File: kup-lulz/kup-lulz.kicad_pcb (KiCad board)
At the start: 4 copper layers, 144.5 x 137 mm, 229 parts, among them J1 CONN_PCIE_PWR_8PIN, J10 SFP_CAGE, J11 CONN_SFP_HOST, J12 SFP_CAGE, J13 PMOD_HOST, J14 PMOD_HOST, J15 CONN_QSFP_HOST, J16 CONN_QSFP_HOST, J17 SMPM, J18 SMPM, J19 SMPM, J2 CONN_IBC_MGMT, J20 SMPM, J21 SMPM, J22 SMPM, J23 SMPM, J24 SMPM, J25 SMPM, J26 SMPM, J27 SMPM, J28 SMPM, J29 SMPM, J3 CONN_01X03, J30 SMPM, J31 SMPM, J32 SMPM, J33 CONN_SFP_HOST, J34 SFP_CAGE, J35 QSFP_CAGE, J36 QSFP_CAGE, J4 CONN_01X05, J7 CONN_SFP_HOST, J8 SFP_CAGE, J9 CONN_SFP_HOST, M1 HEATSINK, M2 SCREWHOLE, M3 SCREWHOLE, M4 SCREWHOLE, M5 SCREWHOLE, SW1 SWITCH, SW2 SWITCH, U1 STM32L031C6U6, U2 MYMGK1R812ERSR, U3 MYMGK1R812ERSR, U4 MYMGK00506ERSR, U5 MYMGK00504ERSR, U6 MYMGK00504ERSR, U7 MYMGK00504ERSR, U9 XILINX_ULTRASCALEPLUS_B676

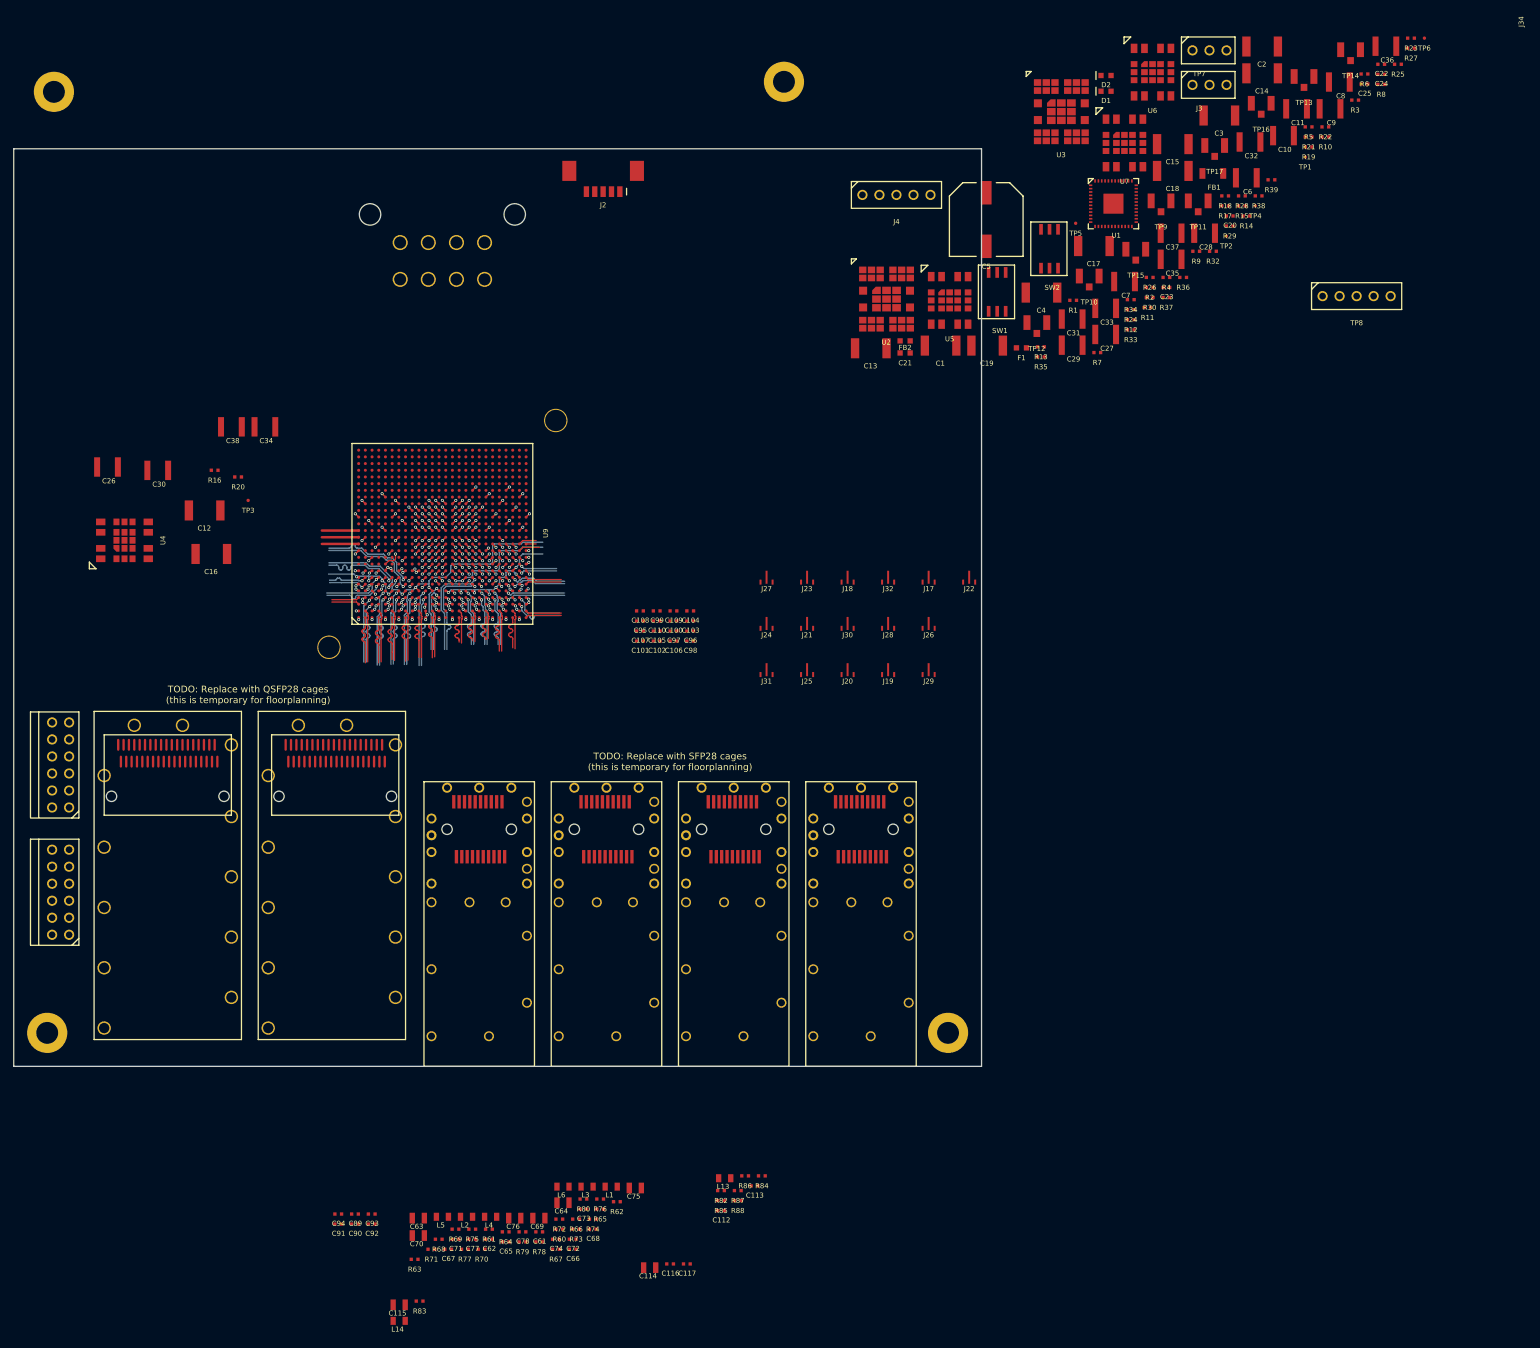
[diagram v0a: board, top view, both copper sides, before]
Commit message: Continued initial work on kup-lulz devboard
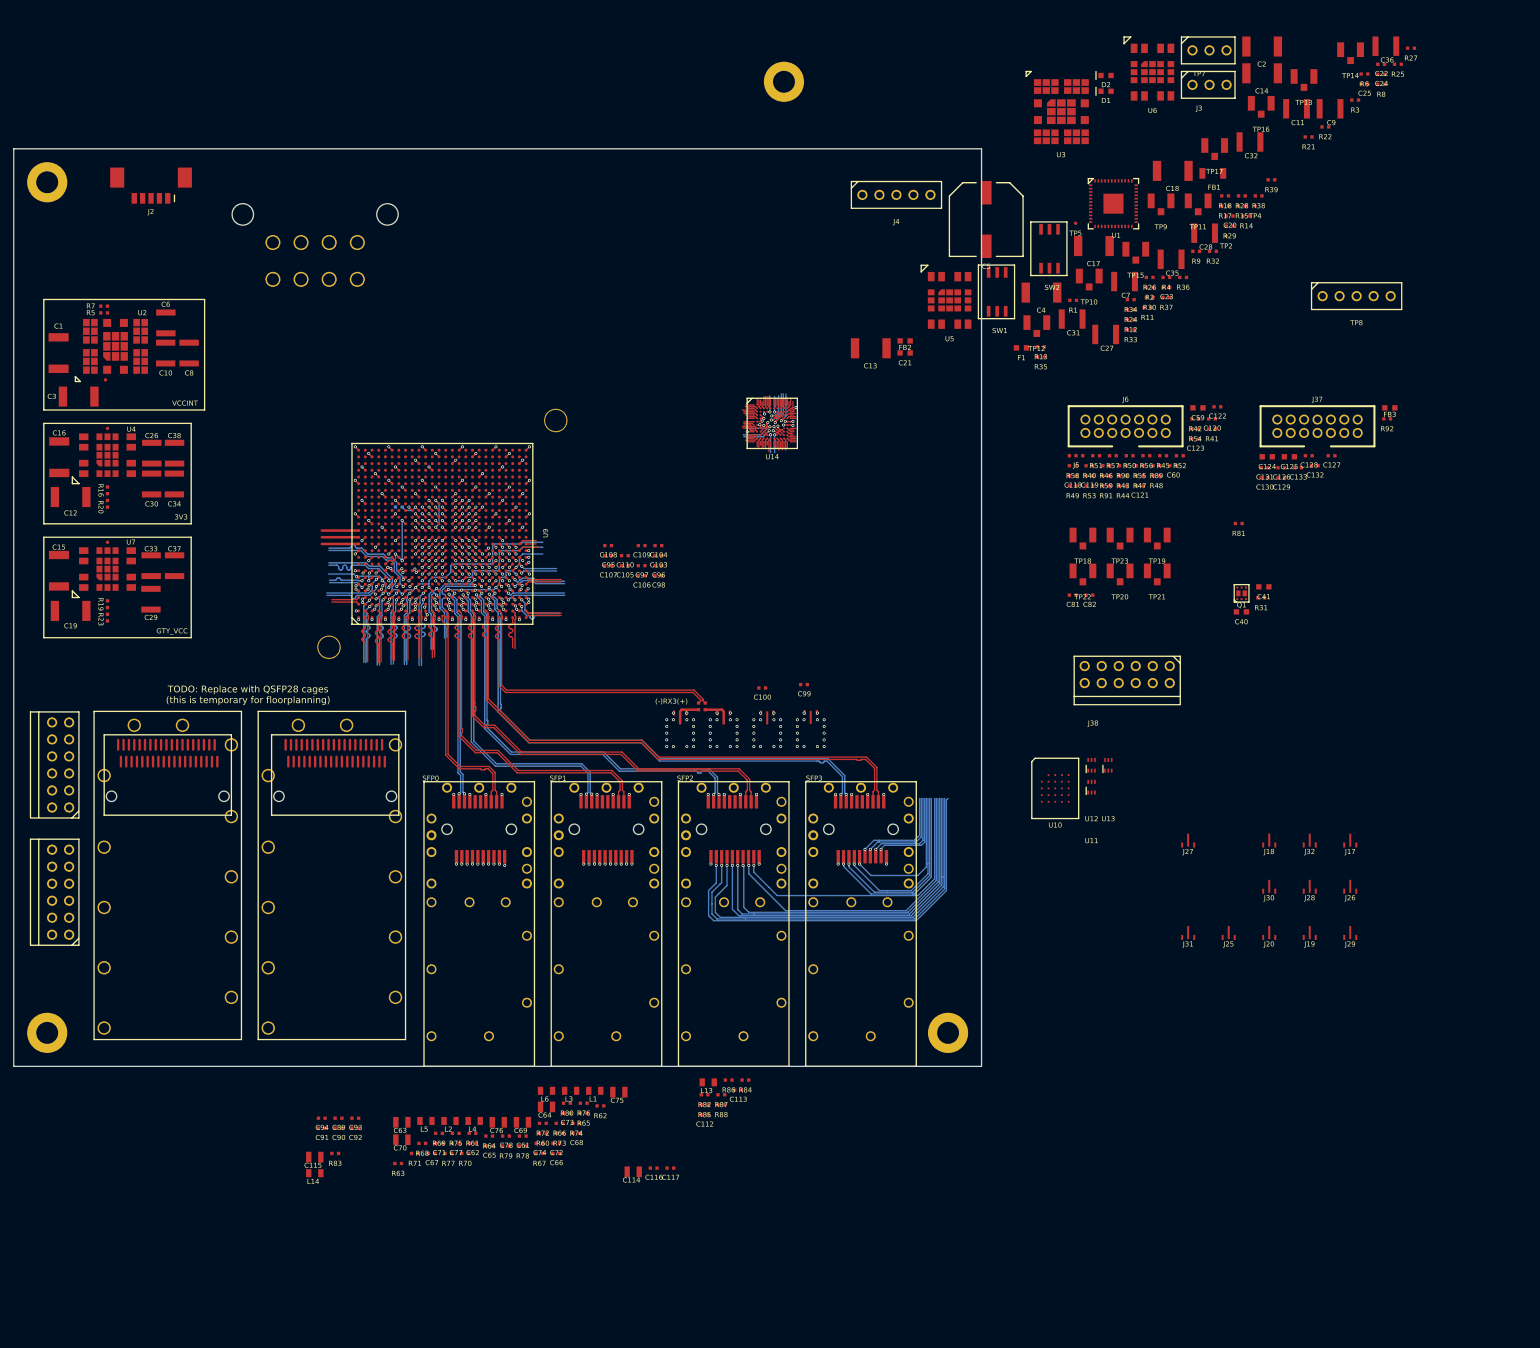
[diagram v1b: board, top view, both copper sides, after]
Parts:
- added C118: 0.47 uF, azonenberg_pcb:EIA_0402_CAP_NOSILK, F.Cu at (208.6, 82.8)
- added C119: 0.47 uF, azonenberg_pcb:EIA_0402_CAP_NOSILK, F.Cu at (211.1, 82.8)
- added C120: 0.47 uF, azonenberg_pcb:EIA_0402_CAP_NOSILK, F.Cu at (229.4, 74.3)
- added C121: 0.47 uF, azonenberg_pcb:EIA_0402_CAP_NOSILK, F.Cu at (218.6, 84.3)
- added C122: 0.47 uF, azonenberg_pcb:EIA_0402_CAP_NOSILK, F.Cu at (230.2, 72.5)
- added C123: 0.47 uF, azonenberg_pcb:EIA_0402_CAP_NOSILK, F.Cu at (226.9, 77.3)
- added C124: 4.7 uF, azonenberg_pcb:EIA_0603_CAP_NOSILK, F.Cu at (237.7, 80.0)
- added C125: 4.7 uF, azonenberg_pcb:EIA_0603_CAP_NOSILK, F.Cu at (241.0, 80.0)
- added C126: 0.47 uF, azonenberg_pcb:EIA_0402_CAP_NOSILK, F.Cu at (239.8, 81.6)
- added C127: 0.47 uF, azonenberg_pcb:EIA_0402_CAP_NOSILK, F.Cu at (247.3, 79.8)
- added C128: 0.47 uF, azonenberg_pcb:EIA_0402_CAP_NOSILK, F.Cu at (243.9, 79.8)
- added C129: 0.47 uF, azonenberg_pcb:EIA_0402_CAP_NOSILK, F.Cu at (239.8, 83.1)
- added C130: 0.47 uF, azonenberg_pcb:EIA_0402_CAP_NOSILK, F.Cu at (237.3, 83.1)
- added C131: 0.47 uF, azonenberg_pcb:EIA_0402_CAP_NOSILK, F.Cu at (237.3, 81.6)
- added C132: 0.47 uF, azonenberg_pcb:EIA_0402_CAP_NOSILK, F.Cu at (244.8, 81.3)
- added C133: 0.47 uF, azonenberg_pcb:EIA_0402_CAP_NOSILK, F.Cu at (242.3, 81.6)
- added C40: 4.7 uF, azonenberg_pcb:EIA_0603_CAP_NOSILK, F.Cu at (233.8, 103.2)
- added C41: 4.7 uF, azonenberg_pcb:EIA_0603_CAP_NOSILK, F.Cu at (237.2, 99.4)
- added C59: 4.7 uF, azonenberg_pcb:EIA_0603_CAP_NOSILK, F.Cu at (227.3, 72.7)
- added C60: 0.47 uF, azonenberg_pcb:EIA_0402_CAP_NOSILK, F.Cu at (223.6, 81.3)
- added C81: 0.1 uF, azonenberg_pcb:EIA_0402_CAP_NOSILK, F.Cu at (208.6, 100.7)
- added C82: 0.1 uF, azonenberg_pcb:EIA_0402_CAP_NOSILK, F.Cu at (211.1, 100.7)
- added FB3: MI0603J601R-10, azonenberg_pcb:EIA_0603_INDUCTOR_NOSILK, F.Cu at (256.0, 72.7)
- added J37: XILINX_JTAG, azonenberg_pcb:XILINX_JTAG_PTH_MOLEX_0878311420, F.Cu at (245.2, 75.4)
- added J38: PMOD_HOST, azonenberg_pcb:CONN_HEADER_2.54MM_2x6_RA_PMOD_HOST, F.Cu at (216.8, 112.5)
- added J5: JUMPER_0402, azonenberg_pcb:EIA_0402_JUMPER, F.Cu at (209.1, 79.8)
- added J6: XILINX_JTAG, azonenberg_pcb:XILINX_JTAG_PTH_MOLEX_0878311420, F.Cu at (216.5, 75.4)
- added Q1: SSM6N58NU, azonenberg_pcb:DFN_6_0.65MM_2x2MM_GDS, F.Cu at (233.8, 100.4)
- added R31: 1K, azonenberg_pcb:EIA_0402_RES_NOSILK, F.Cu at (236.8, 101.0)
- added R40: 0, azonenberg_pcb:EIA_0402_RES_NOSILK, F.Cu at (211.1, 81.3)
- added R41: 0, azonenberg_pcb:EIA_0402_RES_NOSILK, F.Cu at (229.4, 75.8)
- added R42: 0, azonenberg_pcb:EIA_0402_RES_NOSILK, F.Cu at (226.9, 74.3)
- added R43: 4.7K, azonenberg_pcb:EIA_0402_RES_NOSILK, F.Cu at (216.1, 82.8)
- added R44: 33, azonenberg_pcb:EIA_0402_RES_NOSILK, F.Cu at (216.1, 84.3)
- added R45: 33, azonenberg_pcb:EIA_0402_RES_NOSILK, F.Cu at (222.1, 79.8)
- added R46: 33, azonenberg_pcb:EIA_0402_RES_NOSILK, F.Cu at (213.6, 81.3)
- added R47: 33, azonenberg_pcb:EIA_0402_RES_NOSILK, F.Cu at (218.6, 82.8)
- added R48: 33, azonenberg_pcb:EIA_0402_RES_NOSILK, F.Cu at (221.1, 82.8)
- added R49: 33, azonenberg_pcb:EIA_0402_RES_NOSILK, F.Cu at (208.6, 84.3)
- added R50: 33, azonenberg_pcb:EIA_0402_RES_NOSILK, F.Cu at (217.1, 79.8)
- added R51: 33, azonenberg_pcb:EIA_0402_RES_NOSILK, F.Cu at (212.1, 79.8)
- added R52: 33, azonenberg_pcb:EIA_0402_RES_NOSILK, F.Cu at (224.6, 79.8)
- added R53: 33, azonenberg_pcb:EIA_0402_RES_NOSILK, F.Cu at (211.1, 84.3)
- added R54: 33, azonenberg_pcb:EIA_0402_RES_NOSILK, F.Cu at (226.9, 75.8)
- added R55: 4.7K, azonenberg_pcb:EIA_0402_RES_NOSILK, F.Cu at (218.6, 81.3)
- added R56: 4.7K, azonenberg_pcb:EIA_0402_RES_NOSILK, F.Cu at (219.6, 79.8)
- added R57: 4.7K, azonenberg_pcb:EIA_0402_RES_NOSILK, F.Cu at (214.6, 79.8)
- added R58: 4.7K, azonenberg_pcb:EIA_0402_RES_NOSILK, F.Cu at (208.6, 81.3)
- added R59: 4.7K, azonenberg_pcb:EIA_0402_RES_NOSILK, F.Cu at (213.6, 82.8)
- added R81: 100, azonenberg_pcb:EIA_0402_RES_NOSILK, F.Cu at (233.4, 90.0)
- added R89: 4.7K, azonenberg_pcb:EIA_0402_RES_NOSILK, F.Cu at (221.1, 81.3)
- added R90: 4.7K, azonenberg_pcb:EIA_0402_RES_NOSILK, F.Cu at (216.1, 81.3)
- added R91: 4.7K, azonenberg_pcb:EIA_0402_RES_NOSILK, F.Cu at (213.6, 84.3)
- added R92: 33, azonenberg_pcb:EIA_0402_RES_NOSILK, F.Cu at (255.6, 74.3)
- added TP18: U.FL, azonenberg_pcb:CONN_U.FL_TE_1909763-1, F.Cu at (210.1, 91.8)
- added TP19: U.FL, azonenberg_pcb:CONN_U.FL_TE_1909763-1, F.Cu at (221.2, 91.8)
- added TP20: U.FL, azonenberg_pcb:CONN_U.FL_TE_1909763-1, F.Cu at (215.7, 97.1)
- added TP21: U.FL, azonenberg_pcb:CONN_U.FL_TE_1909763-1, F.Cu at (221.2, 97.1)
- added TP22: U.FL, azonenberg_pcb:CONN_U.FL_TE_1909763-1, F.Cu at (210.1, 97.1)
- added TP23: U.FL, azonenberg_pcb:CONN_U.FL_TE_1909763-1, F.Cu at (215.7, 91.8)
- added U10: MT25QU256ABA8E12-0AUT, azonenberg_pcb:BGA_24_6x8_DEPOP1_1MM, F.Cu at (206.0, 129.5)
- added U11: 74LVC1T45, azonenberg_pcb:DFN_6_0.5MM_1.6x1.6MM_TI_DPK, F.Cu at (211.4, 129.3)
- added U12: 74LVC1T45, azonenberg_pcb:DFN_6_0.5MM_1.6x1.6MM_TI_DPK, F.Cu at (211.4, 126.0)
- added U13: 74LVC1T45, azonenberg_pcb:DFN_6_0.5MM_1.6x1.6MM_TI_DPK, F.Cu at (213.9, 126.0)
- added U14: STM32L431VxIx, azonenberg_pcb:BGA_100_7x7_DEPOP_0.5MM_STM32_UFBGA100_OSHPARK, F.Cu at (163.8, 75.0)
- R10: moved to B.Cu
- moved R23 213.0 mm to (64.5, 104.0), turned to 90 degrees
- moved TP6 210.5 mm to (64.5, 92.8)
- moved R19 191.9 mm to (64.5, 102.0), turned to -90 degrees
- moved TP1 182.2 mm to (64.2, 68.5)
- moved R5 182.0 mm to (64.0, 58.5), turned to 180 degrees
- moved C15 178.1 mm to (57.2, 97.0), turned to 90 degrees
- moved C8 176.4 mm to (76.7, 64.5), turned to -90 degrees
- moved C3 175.4 mm to (60.2, 71.0), turned to 180 degrees
- moved C10 170.0 mm to (73.2, 64.5), turned to -90 degrees
- moved U7 164.6 mm to (64.5, 96.8), turned to 90 degrees
- moved C6 162.8 mm to (73.2, 60.0), turned to 90 degrees
- moved C37 156.9 mm to (74.5, 96.2), turned to 90 degrees
- moved R10 149.0 mm to (108.0, 87.5)
- moved R7 148.4 mm to (64.0, 57.5)
- moved C33 147.6 mm to (71.0, 96.2), turned to 90 degrees
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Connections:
- net /Power Supply/12V0 renamed /12V0
- net /Power Supply/2V5 renamed /2V5
- net /Power Supply/3V3_SB renamed /3V3_SB
- net /SFP28 interfaces/3V3 renamed /3V3
- C112 pad 2: /SFP28 interfaces/GND -> /GND
- C113 pad 2: /SFP28 interfaces/GND -> /GND
- C116 pad 2: /SFP28 interfaces/GND -> /GND
- C117 pad 2: /SFP28 interfaces/GND -> /GND
- C61 pad 2: /SFP28 interfaces/GND -> /GND
- C62 pad 2: /SFP28 interfaces/GND -> /GND
- C65 pad 2: /SFP28 interfaces/GND -> /GND
- C66 pad 2: /SFP28 interfaces/GND -> /GND
- C67 pad 2: /SFP28 interfaces/GND -> /GND
- C68 pad 2: /SFP28 interfaces/GND -> /GND
- C71 pad 2: /SFP28 interfaces/GND -> /GND
- C72 pad 2: /SFP28 interfaces/GND -> /GND
- C73 pad 2: /SFP28 interfaces/GND -> /GND
- C74 pad 2: /SFP28 interfaces/GND -> /GND
- C77 pad 2: /SFP28 interfaces/GND -> /GND
- C78 pad 2: /SFP28 interfaces/GND -> /GND
- J10 pad 1: /SFP28 interfaces/GND -> /GND
- J11 pad 1: /SFP28 interfaces/GND -> /GND
- J11 pad 10: /SFP28 interfaces/GND -> /GND
- J11 pad 11: /SFP28 interfaces/GND -> /GND
- J11 pad 12: /SFP28 interfaces/SFP0_RX_N -> /SFP28 interfaces/SFP0_RX_P
- J11 pad 13: /SFP28 interfaces/SFP0_RX_P -> /SFP28 interfaces/SFP0_RX_N
- J11 pad 14: /SFP28 interfaces/GND -> /GND
- J11 pad 17: /SFP28 interfaces/GND -> /GND
- J11 pad 20: /SFP28 interfaces/GND -> /GND
- J12 pad 1: /SFP28 interfaces/GND -> /GND
- J17 pad 2: /SMPM ports/GND -> /GND
- J18 pad 2: /SMPM ports/GND -> /GND
- J19 pad 2: /SMPM ports/GND -> /GND
- J20 pad 2: /SMPM ports/GND -> /GND
- J21 pad 2: /SMPM ports/GND -> /GND
- J22 pad 2: /SMPM ports/GND -> /GND
- J23 pad 2: /SMPM ports/GND -> /GND
- J24 pad 2: /SMPM ports/GND -> /GND
- J25 pad 2: /SMPM ports/GND -> /GND
- J26 pad 2: /SMPM ports/GND -> /GND
- J27 pad 2: /SMPM ports/GND -> /GND
- J28 pad 2: /SMPM ports/GND -> /GND
- J29 pad 2: /SMPM ports/GND -> /GND
- J30 pad 2: /SMPM ports/GND -> /GND
- J31 pad 2: /SMPM ports/GND -> /GND
- J32 pad 2: /SMPM ports/GND -> /GND
- J33 pad 1: /SFP28 interfaces/GND -> /GND
- J33 pad 10: /SFP28 interfaces/GND -> /GND
- J33 pad 11: /SFP28 interfaces/GND -> /GND
- J33 pad 12: /SFP28 interfaces/SFP3_RX_N -> /SFP28 interfaces/SFP3_RX_P
- J33 pad 13: /SFP28 interfaces/SFP3_RX_P -> /SFP28 interfaces/SFP3_RX_N
- J33 pad 14: /SFP28 interfaces/GND -> /GND
- J33 pad 17: /SFP28 interfaces/GND -> /GND
- J33 pad 20: /SFP28 interfaces/GND -> /GND
- J34 pad 1: /SFP28 interfaces/GND -> /GND
- J7 pad 1: /SFP28 interfaces/GND -> /GND
- J7 pad 10: /SFP28 interfaces/GND -> /GND
- J7 pad 11: /SFP28 interfaces/GND -> /GND
- J7 pad 12: /SFP28 interfaces/SFP2_RX_N -> /SFP28 interfaces/SFP2_RX_P
- J7 pad 13: /SFP28 interfaces/SFP2_RX_P -> /SFP28 interfaces/SFP2_RX_N
- J7 pad 14: /SFP28 interfaces/GND -> /GND
- J7 pad 17: /SFP28 interfaces/GND -> /GND
- J7 pad 20: /SFP28 interfaces/GND -> /GND
- J8 pad 1: /SFP28 interfaces/GND -> /GND
- J9 pad 1: /SFP28 interfaces/GND -> /GND
- J9 pad 10: /SFP28 interfaces/GND -> /GND
- J9 pad 11: /SFP28 interfaces/GND -> /GND
- J9 pad 12: /SFP28 interfaces/SFP1_RX_N -> /SFP28 interfaces/SFP1_RX_P
- J9 pad 13: /SFP28 interfaces/SFP1_RX_P -> /SFP28 interfaces/SFP1_RX_N
- J9 pad 14: /SFP28 interfaces/GND -> /GND
- J9 pad 17: /SFP28 interfaces/GND -> /GND
- J9 pad 20: /SFP28 interfaces/GND -> /GND
- R63 pad 1: /SFP28 interfaces/GND -> /GND
- R64 pad 1: /SFP28 interfaces/GND -> /GND
- R70 pad 1: /SFP28 interfaces/GND -> /GND
- R71 pad 1: /SFP28 interfaces/GND -> /GND
- R77 pad 1: /SFP28 interfaces/GND -> /GND
- R78 pad 1: /SFP28 interfaces/GND -> /GND
- R85 pad 1: /SFP28 interfaces/GND -> /GND
- R86 pad 1: /SFP28 interfaces/GND -> /GND
- U1 pad 11: /Power Supply/FPGA_RST_N -> /FPGA support/FPGA_RESET_N_3V3
- U1 pad 22: /Power Supply/FPGA_DONE -> /FPGA support/FPGA_DONE_3V3
- U1 pad 25: /Power Supply/FPGA_INIT -> /FPGA support/FPGA_INIT_3V3
- U4 pad 5: /FPGA support/1V8 -> /FPGA support/3V3
- U9 pad AA4: /SFP28 interfaces/SFP0_TX_N -> /SFP28 interfaces/SFP3_TX_N
- U9 pad AA5: /SFP28 interfaces/SFP0_TX_P -> /SFP28 interfaces/SFP3_TX_P
- U9 pad AB6: /SMPM ports/K_REFCLK_0_N -> unconnected-(U9-PadAB6)
- U9 pad AB7: /SMPM ports/K_REFCLK_0_P -> unconnected-(U9-PadAB7)
- U9 pad K6: /QSFP28 interface/QSFP28A_REFCLK0_N -> unconnected-(U9-PadK6)
- U9 pad K7: /QSFP28 interface/QSFP28A_REFCLK0_P -> unconnected-(U9-PadK7)
- U9 pad M6: /QSFP28 interface/QSFP28B_REFCLK1_N -> unconnected-(U9-PadM6)
- U9 pad M7: /QSFP28 interface/QSFP28B_REFCLK1_P -> unconnected-(U9-PadM7)
- U9 pad P1: /SFP28 interfaces/SFP3_RX_N -> /SFP28 interfaces/SFP0_RX_N
- U9 pad P2: /SFP28 interfaces/SFP3_RX_P -> /SFP28 interfaces/SFP0_RX_P
- U9 pad P6: /QSFP28 interface/QSFP28B_REFCLK0_N -> unconnected-(U9-PadP6)
- U9 pad P7: /QSFP28 interface/QSFP28B_REFCLK0_P -> unconnected-(U9-PadP7)
- U9 pad R4: /SFP28 interfaces/SFP3_TX_N -> /SFP28 interfaces/SFP0_TX_N
- U9 pad R5: /SFP28 interfaces/SFP3_TX_P -> /SFP28 interfaces/SFP0_TX_P
- U9 pad T1: /SFP28 interfaces/SFP2_RX_N -> /SFP28 interfaces/SFP1_RX_N
- U9 pad T2: /SFP28 interfaces/SFP2_RX_P -> /SFP28 interfaces/SFP1_RX_P
- U9 pad T6: /SFP28 interfaces/SFP28_REFCLK1_N -> unconnected-(U9-PadT6)
- U9 pad T7: /SFP28 interfaces/SFP28_REFCLK1_P -> unconnected-(U9-PadT7)
- U9 pad U4: /SFP28 interfaces/SFP2_TX_N -> /SFP28 interfaces/SFP1_TX_N
- U9 pad U5: /SFP28 interfaces/SFP2_TX_P -> /SFP28 interfaces/SFP1_TX_P
- U9 pad V1: /SFP28 interfaces/SFP1_RX_N -> /SFP28 interfaces/SFP2_RX_N
- U9 pad V2: /SFP28 interfaces/SFP1_RX_P -> /SFP28 interfaces/SFP2_RX_P
- U9 pad W4: /SFP28 interfaces/SFP1_TX_N -> /SFP28 interfaces/SFP2_TX_N
- U9 pad W5: /SFP28 interfaces/SFP1_TX_P -> /SFP28 interfaces/SFP2_TX_P
- U9 pad Y1: /SFP28 interfaces/SFP0_RX_N -> /SFP28 interfaces/SFP3_RX_N
- U9 pad Y2: /SFP28 interfaces/SFP0_RX_P -> /SFP28 interfaces/SFP3_RX_P
- U9 pad Y6: /SMPM ports/K_REFCLK_1_N -> unconnected-(U9-PadY6)
- U9 pad Y7: /SMPM ports/K_REFCLK_1_P -> unconnected-(U9-PadY7)
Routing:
- net /GND: track 0.00 -> 595.4 mm, vias 0 -> 89
- net /FPGA support/3V3: track 35.6 -> 337.4 mm
- net /FPGA support/GND: track 347.6 -> 528.9 mm, vias 175 -> 203
- net /SFP28 interfaces/SFP3_RX_P: track 0.00 -> 80.8 mm
- net /SFP28 interfaces/SFP3_RX_N: track 0.00 -> 80.8 mm
- net /SFP28 interfaces/SFP3_TX_N: track 0.49 -> 78.4 mm, vias 1 -> 2
- net /SFP28 interfaces/SFP3_TX_P: track 0.49 -> 78.4 mm, vias 1 -> 2
- net /SFP28 interfaces/SFP2_TX_FAULT: track 0.00 -> 60.8 mm, vias 0 -> 1
- net /SFP28 interfaces/SFP2_TX_DISABLE: track 0.00 -> 59.6 mm, vias 0 -> 1
- net /SFP28 interfaces/SFP2_RX_P: track 5.03 -> 64.4 mm
- net /SFP28 interfaces/SFP2_RX_N: track 4.93 -> 64.3 mm
- net /SFP28 interfaces/SFP2_I2C_SDA: track 0.00 -> 58.4 mm, vias 0 -> 1
- net /SFP28 interfaces/SFP2_I2C_SCL: track 0.00 -> 54.3 mm, vias 0 -> 1
- net /SFP28 interfaces/SFP2_TX_P: track 8.59 -> 62.5 mm, vias 1 -> 2
- net /SFP28 interfaces/SFP2_TX_N: track 8.55 -> 62.4 mm, vias 1 -> 2
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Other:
- board text added: "(-)RX3(+)"
- board text added: "3V3"
- board text added: "GTY_VCC"
- board text added: "SFP0"
- board text added: "SFP1"
- board text added: "SFP2"
- board text added: "SFP3"
- board text added: "VCCINT"
- board text removed: "TODO: Replace with SFP28 cages (this is temporary for floorplanning)"
